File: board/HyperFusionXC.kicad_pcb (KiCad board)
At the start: 2 copper layers, 102 x 65.5 mm, 142 parts, among them J1 Conn_01x02_Pin, J2 10067847-001RLF, J3 UJ20-C-H-G-SMT-2-P16-TR, J4 UJ20-C-H-G-SMT-2-P16-TR, J5 Conn_01x08, J6 Conn_01x05, J7 Conn_02x05_Odd_Even, Q1 UM6K34NTCN, U1 SOM_FPGA_LP, U10 SN74LVC1G04DCKR, U11 AP22816BKAWT-7, U12 TXS0108EPWR, U14 TXS0108EPWR, U15 TXB0104D, U2 74AHC541, U3 74AHC541, U4 MAX3814, U5 NAU88C22A, U6 ESP32-S3-WROOM-1-N8R8, U7 MCP2221AT-I/SL, U8 74AHC541, U9 AP22816BKAWT-7, X1 EDGE50/MSX, X2 SS-53000-001, X3 490107671012_JTAG

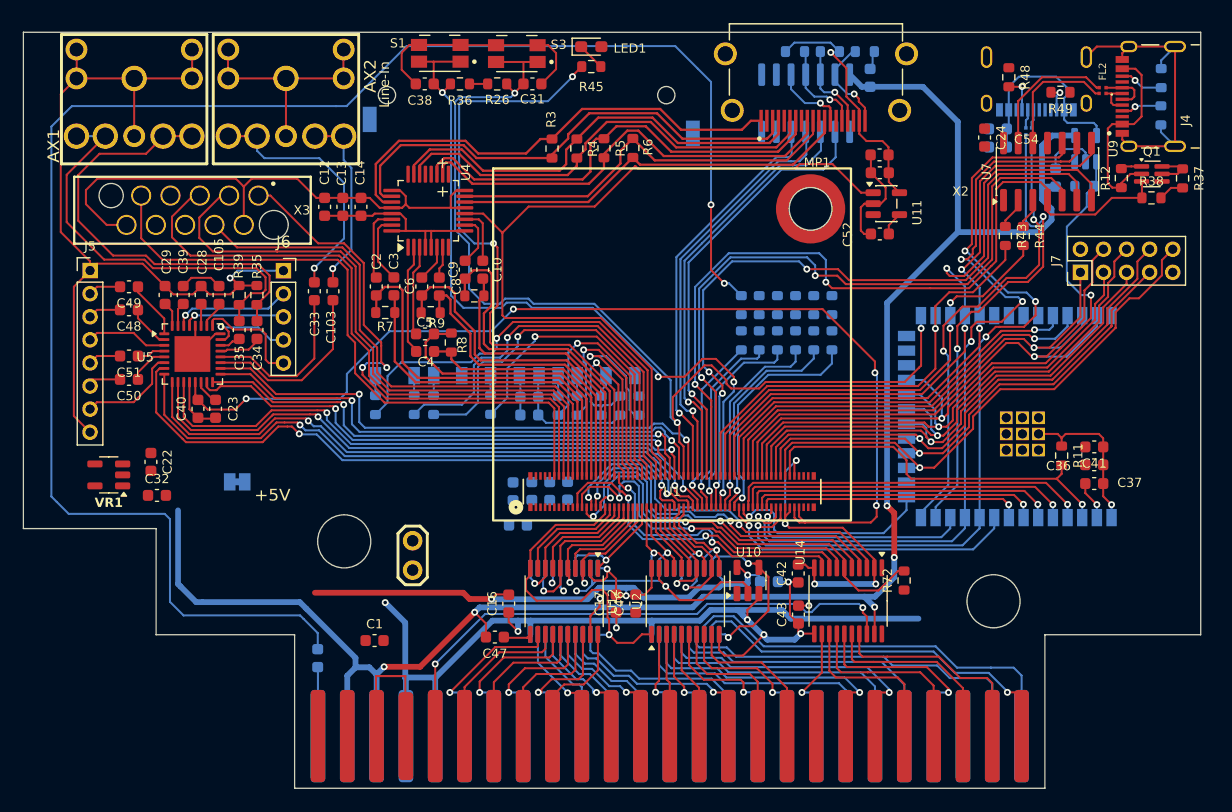
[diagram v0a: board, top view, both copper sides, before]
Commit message: PCB work in progress
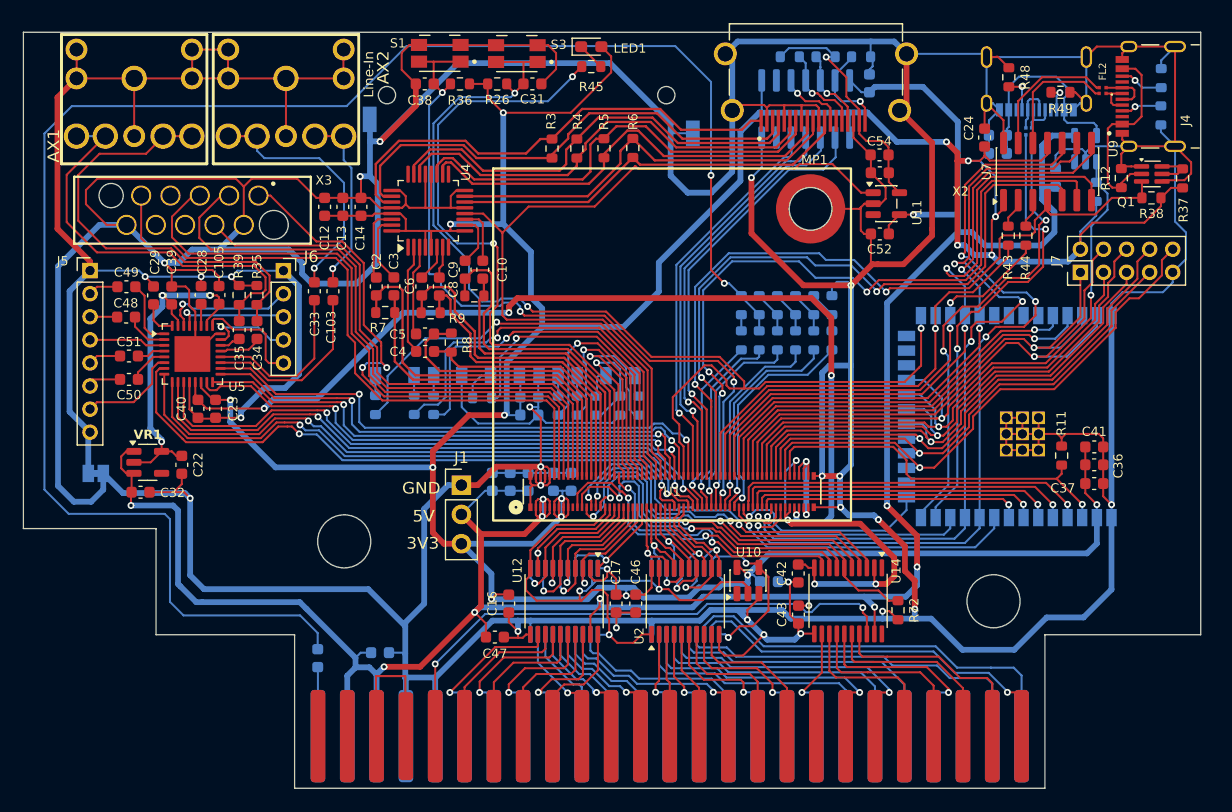
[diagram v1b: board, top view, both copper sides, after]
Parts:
- C1: moved to B.Cu
- J1: value Conn_01x02_Pin -> Conn_01x03; footprint Library:JUMPER_1 -> Connector_PinHeader_2.54mm:PinHeader_1x03_P2.54mm_Vertical
- U1: value SOM_FPGA_LP -> CONN_DF40C-120DP-0p4V51_120P_HIR
- moved R99 12.3 mm to (99.3, 107.7)
- moved J1 6.41 mm to (130.9, 108.7), turned to 0 degrees
- moved C30 4.36 mm to (133.6, 108.5), turned to 90 degrees
- moved VR1 3.55 mm to (103.8, 106.8), turned to 0 degrees
- moved C22 2.69 mm to (106.7, 107.0), turned to 90 degrees
- moved R72 2.63 mm to (168.8, 119.6)
- moved C32 1.45 mm to (103.2, 109.3)
- moved C1 1.15 mm to (123.9, 123.2), turned to 180 degrees
- moved R50 1.14 mm to (185.9, 83.3), turned to -90 degrees
- moved C29 1.00 mm to (104.3, 92.3)
- moved C39 1.00 mm to (105.8, 92.3)
- moved R29 0.94 mm to (132.8, 101.2), turned to 180 degrees
- moved C11 0.86 mm to (138.9, 108.5), turned to -90 degrees
- moved C20 0.86 mm to (136.7, 108.5), turned to -90 degrees
- moved C44 0.86 mm to (135.2, 108.5), turned to -90 degrees
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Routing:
- net GND: track 247.4 -> 776.0 mm, vias 8 -> 22
- net +3V3: track 88.6 -> 339.5 mm, vias 5 -> 17
- net +5V: track 177.6 -> 232.8 mm, vias 7 -> 11
- net GNDA: track 101.1 -> 129.3 mm, vias 1 -> 4
- net +3V3DAC: track 4.42 -> 30.2 mm, vias 0 -> 3
- net +IO3V3: track 0.00 -> 10.4 mm, vias 0 -> 2
- net +IO1V8: track 90.8 -> 84.3 mm
- net /~{DBG_RST}: track 71.1 -> 66.6 mm
- net /ESP_BOOT_MODE: track 91.1 -> 95.5 mm
- net Net-(C18-Pad2): track 146.8 -> 151.0 mm
- net +IO2V5: track 29.1 -> 32.9 mm
- net Net-(R19-Pad1): track 0.00 -> 3.70 mm
- net Net-(R17-Pad1): track 0.00 -> 3.70 mm
- net Net-(R18-Pad1): track 0.00 -> 3.70 mm
- net Net-(R16-Pad1): track 0.00 -> 3.70 mm
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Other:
- board text added: "3V3"
- board text added: "5V"
- board text added: "GND"
- board text removed: "+"
- board text removed: "+5V"
